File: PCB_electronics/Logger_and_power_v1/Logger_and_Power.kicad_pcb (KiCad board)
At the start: 2 copper layers, 41 parts, among them IC1 ATMEGA328-P, P1 SOLAR_PANEL, P10 CONN_01X08, P11 CONN_01X08, P12 CONN_01X03, P13 CONN_01X02, P14 CONN_01X02, P15 CONN_01X02, P2 5V_pololu, P3 BATT, P4 SUPERCAPS, P5 GPS_breakout_connector, P6 SD_breakout_connector, P7 Iridium_connector, P8 VN100_connector, P9 RPI_connector, U1 IRLB_8721_SOL, U2 IRLS-8721_MEGA, U3 MAX232, U4 FQP27P06, Y1 16MHz

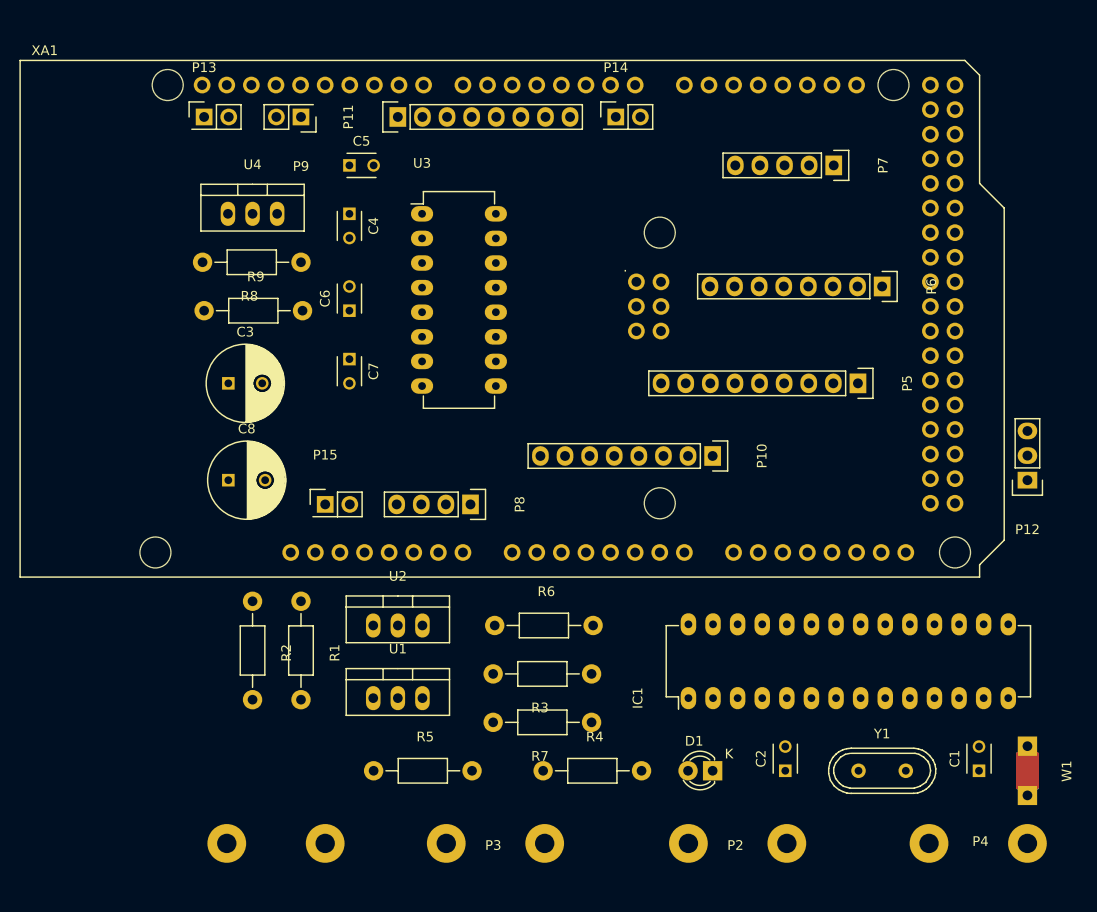
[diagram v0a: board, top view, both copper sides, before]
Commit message: routed ok
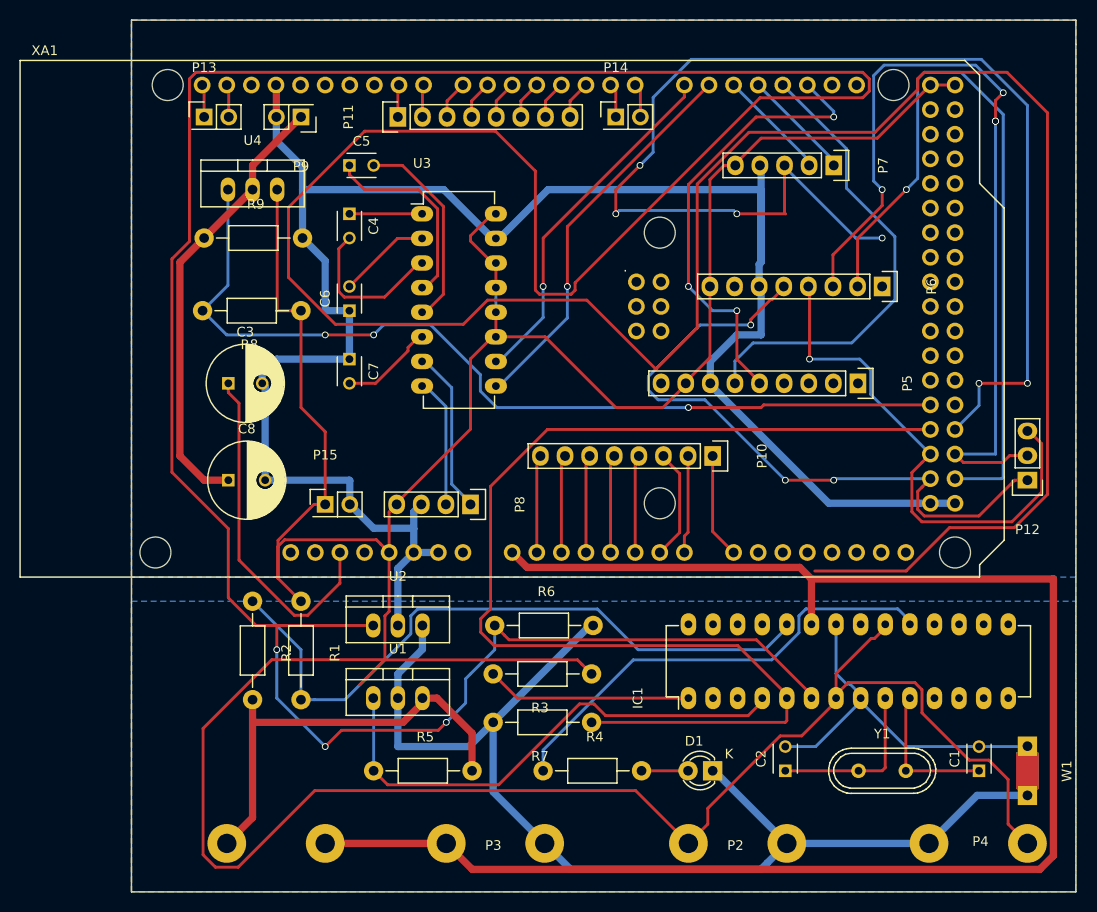
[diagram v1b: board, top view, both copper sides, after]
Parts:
- moved R9 7.50 mm to (167.5, 70.0)
- moved R8 5.00 mm to (177.5, 77.5)
- moved U4 2.50 mm to (172.5, 65.0)
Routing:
- net /Power_part/D5: track 0.00 -> 489.7 mm, vias 0 -> 3
- net +5V: track 0.00 -> 374.9 mm
- net /Power_part/Mega_ground: track 0.00 -> 204.7 mm
- net /Power_part/Batt_plus: track 0.00 -> 167.2 mm
- net /Logger_part/IRD_ON_OFF: track 0.00 -> 131.4 mm, vias 0 -> 6
- net /Power_part/Feedback_Mega: track 0.00 -> 120.5 mm
- net GND: track 0.00 -> 118.5 mm
- net /Logger_part/RPI_control: track 0.00 -> 94.8 mm, vias 0 -> 3
- net /Logger_part/MOSI: track 0.00 -> 89.2 mm, vias 0 -> 4
- net /Logger_part/SS: track 0.00 -> 77.4 mm, vias 0 -> 1
- net /Power_part/A1: track 0.00 -> 70.4 mm
- net /Logger_part/SCK: track 0.00 -> 69.5 mm, vias 0 -> 3
- net /Logger_part/MISO: track 0.00 -> 54.6 mm, vias 0 -> 1
- net /Power_part/D3: track 0.00 -> 53.7 mm
- net /Logger_part/MEGA_TX_1: track 0.00 -> 48.4 mm
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- added copper zone on F.Cu, net +5V
- added copper zone on B.Cu, net /Power_part/Mega_ground
- added copper zone on B.Cu, net GND
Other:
- board outline added: 97.5 x 90 mm
- net class Default: clearance 0.2 -> 0.3; trace_width 0.25 -> 0.3; via_dia 0.6 -> 0.7; via_drill 0.4 -> 0.5
- net class power added: clearance 0.3, trace_width 0.75, via_dia 0.9, via_drill 0.6
- rule trace_clearance: 0.2 -> 0.3
